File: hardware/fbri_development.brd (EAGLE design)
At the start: 50 x 50 mm, 107 parts, among them IC3 TLV70033DCK, U1 SAM_D20E, U2 SI4060, U3 MAX1947, U4 ANTENOVA_GPS_M10382, U5 S25FS-S, U6 STM32F_48PIN, U7 LP38501TS-ADJ/NOPB, Y1 8MHz

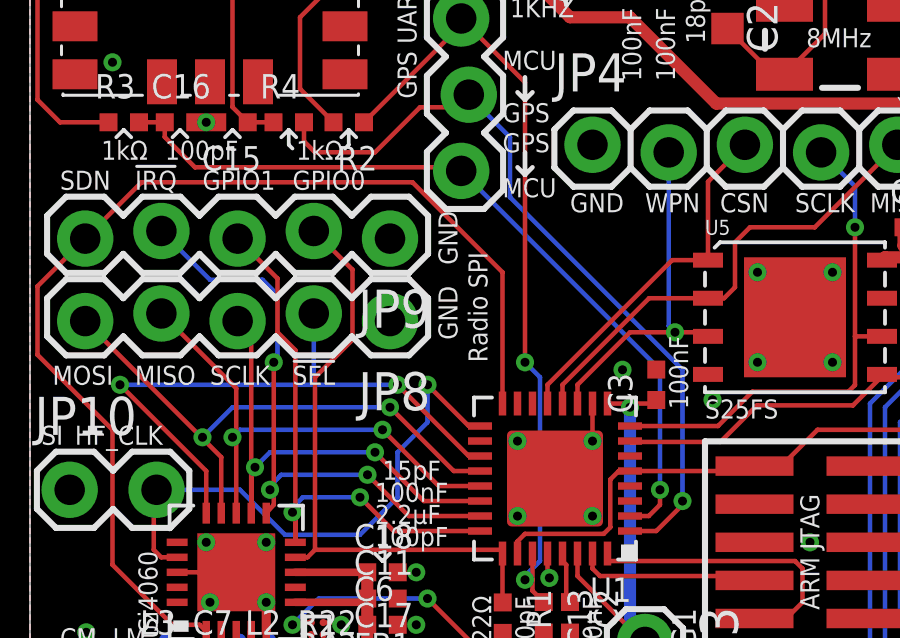
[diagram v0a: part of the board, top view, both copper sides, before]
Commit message: Before rename
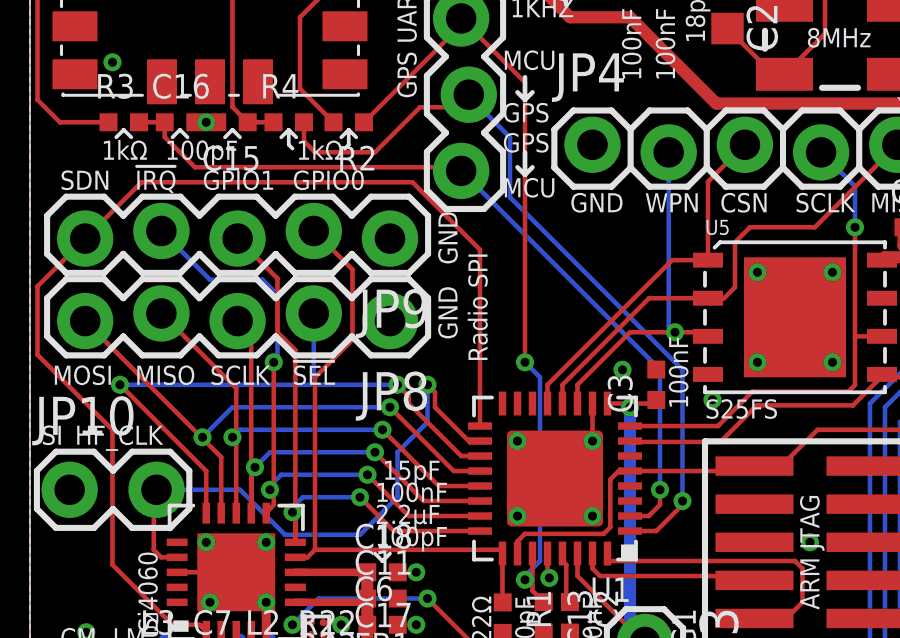
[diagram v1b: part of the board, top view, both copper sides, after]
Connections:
- net SI_HF_CLK: now also U1.18; no longer U1.17
- net SI_SDN: now also U1.17; no longer U1.16
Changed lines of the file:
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@@
 <wire x1="12.25" y1="14.25" x2="9.46" y2="14.25" width="0.1524" layer="16"/>
 <wire x1="9.46" y1="14.25" x2="3" y2="14.25" width="0.1524" layer="16"/>
-<wire x1="15" y1="11.875" x2="14.625" y2="11.875" width="0.1524" layer="1"/>
-<wire x1="14.625" y1="11.875" x2="12.25" y2="14.25" width="0.1524" layer="1"/>
+<wire x1="15" y1="11.875" x2="14.375" y2="11.875" width="0.1524" layer="1"/>
+<wire x1="14.375" y1="11.875" x2="12.625" y2="13.625" width="0.1524" layer="1"/>
+<wire x1="12.625" y1="13.625" x2="12.625" y2="13.875" width="0.1524" layer="1"/>
+<wire x1="12.625" y1="13.875" x2="12.25" y2="14.25" width="0.1524" layer="1"/>
 </signal>
 <signal name="TIME_1KHZ">
@@
 <signal name="SI_HF_CLK">
 <contactref element="U2" pad="17"/>
-<contactref element="U1" pad="17"/>
 <contactref element="JP10" pad="2"/>
 <wire x1="4.905" y1="8.5" x2="4.375" y2="8.5" width="0.1524" layer="1"/>
@@
 <wire x1="12.25" y1="12" x2="13.25" y2="13" width="0.1524" layer="16"/>
 <wire x1="13.25" y1="13" x2="13.25" y2="14.25" width="0.1524" layer="16"/>
-<wire x1="15" y1="12.875" x2="14.625" y2="12.875" width="0.1524" layer="1"/>
-<wire x1="14.625" y1="12.875" x2="13.25" y2="14.25" width="0.1524" layer="1"/>
+<wire x1="14.625" y1="12.375" x2="13.5" y2="13.5" width="0.1524" layer="1"/>
+<wire x1="13.5" y1="13.5" x2="13.5" y2="14" width="0.1524" layer="1"/>
+<wire x1="13.5" y1="14" x2="13.25" y2="14.25" width="0.1524" layer="1"/>
+<contactref element="U1" pad="18"/>
+<wire x1="15" y1="12.375" x2="14.625" y2="12.375" width="0.1524" layer="1"/>
 </signal>
 <signal name="SI_SDN">
-<contactref element="U1" pad="16"/>
 <contactref element="U2" pad="1"/>
 <contactref element="JP9" pad="5"/>
@@
 <wire x1="0.25" y1="15.25" x2="0.25" y2="17.533" width="0.1524" layer="1"/>
 <wire x1="0.25" y1="17.533" x2="1.84" y2="19.123" width="0.1524" layer="1"/>
-<wire x1="15.75" y1="13.625" x2="15.75" y2="18" width="0.1524" layer="1"/>
 <wire x1="12.75" y1="21" x2="3.717" y2="21" width="0.1524" layer="1"/>
 <wire x1="3.717" y1="21" x2="1.84" y2="19.123" width="0.1524" layer="1"/>
-<wire x1="12.75" y1="21" x2="15.75" y2="18" width="0.1524" layer="1"/>
+<wire x1="12.75" y1="21" x2="15" y2="18.75" width="0.1524" layer="1"/>
+<contactref element="U1" pad="17"/>
+<wire x1="15" y1="12.875" x2="15" y2="18.75" width="0.1524" layer="1"/>
 </signal>
 <signal name="SI_GPIO0">
